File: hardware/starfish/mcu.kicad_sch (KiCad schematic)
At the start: 40 parts, among them SW301 RESET, SW302 BOOTSEL, U301 RP2040, U302 W25Q128JVS, Y301 12MHz

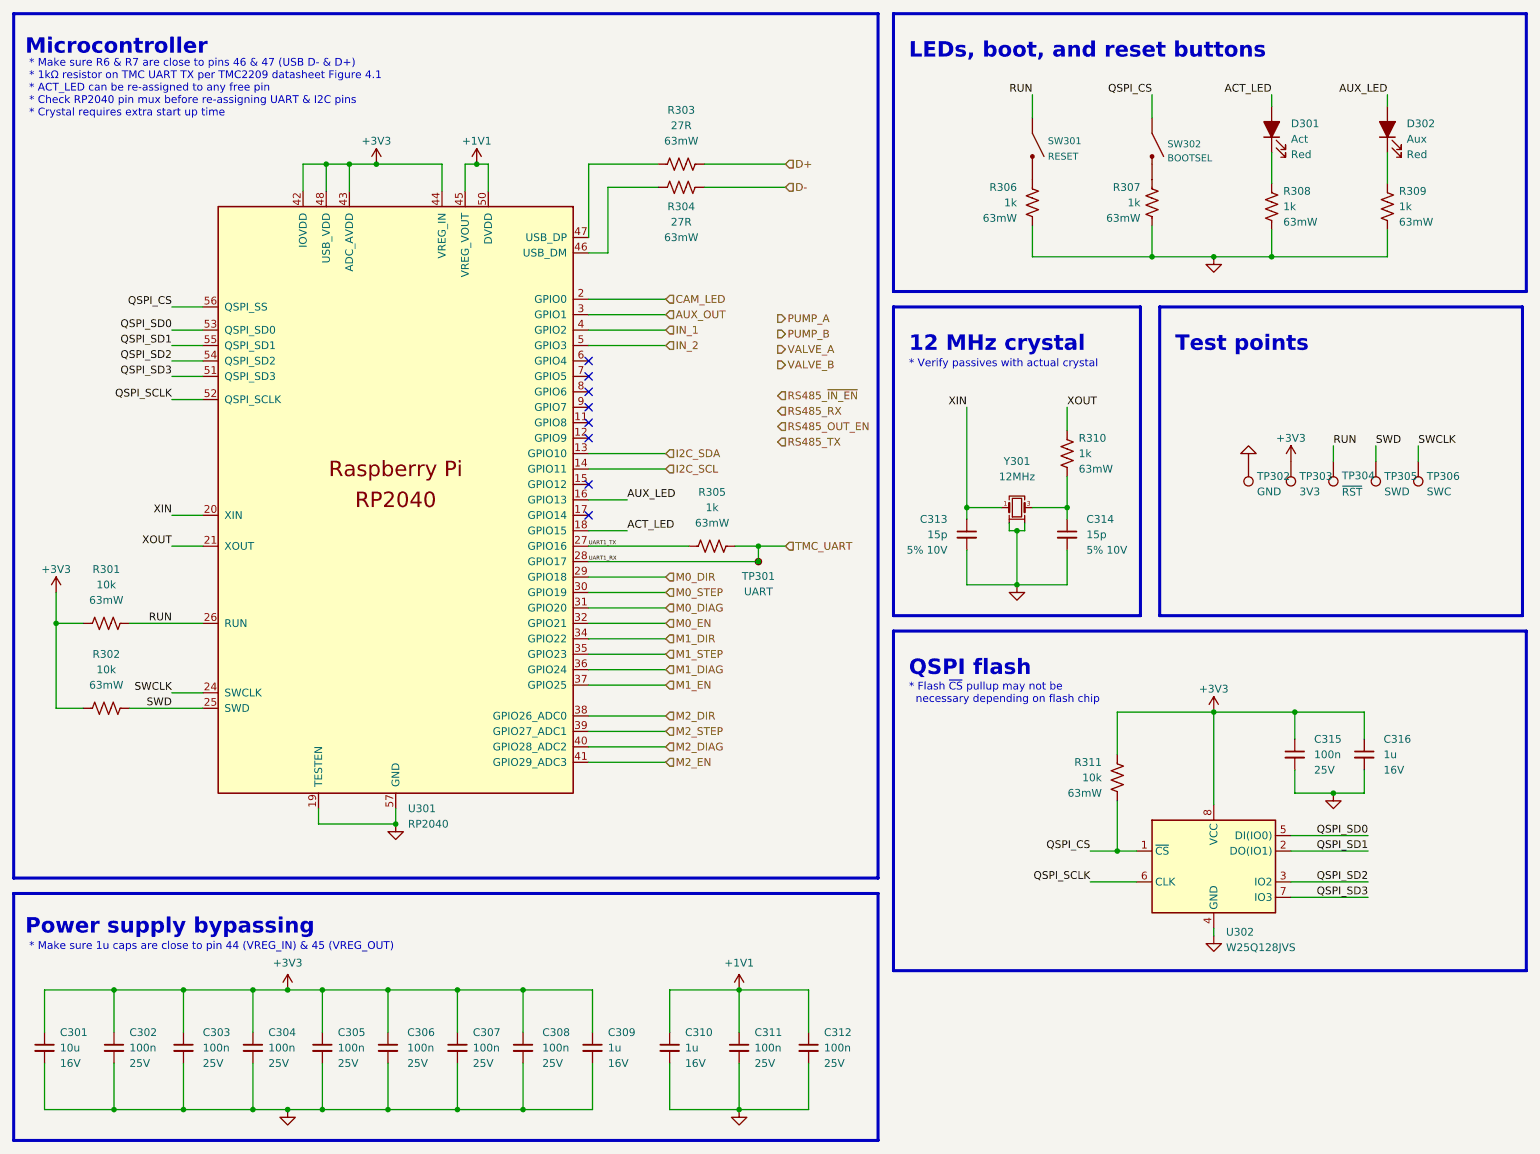
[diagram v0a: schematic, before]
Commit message: First pass at layout and routing
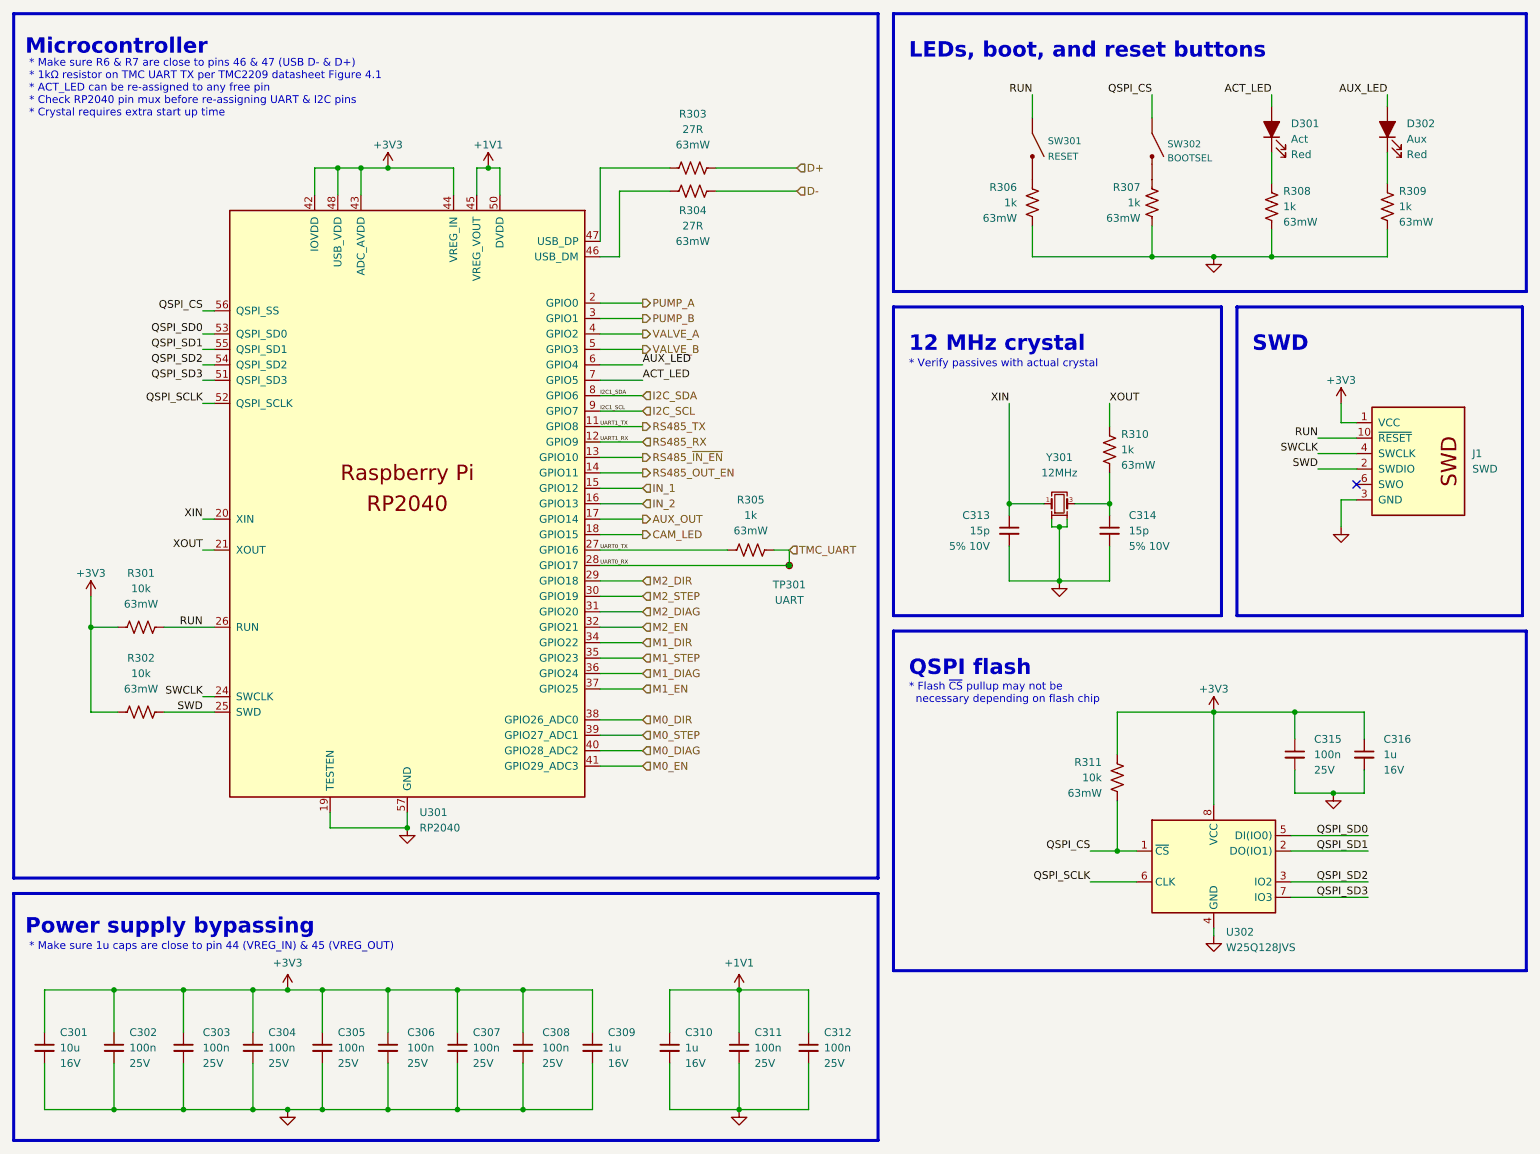
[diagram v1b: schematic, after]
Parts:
- removed TP302: GND, TestPoint:TestPoint_Pad_D1.0mm, symbol Connector:TestPoint
- removed TP303: 3V3, TestPoint:TestPoint_Pad_D1.0mm, symbol Connector:TestPoint
- removed TP304: ~{RST}, TestPoint:TestPoint_Pad_D1.0mm, symbol Connector:TestPoint
- removed TP305: SWD, TestPoint:TestPoint_Pad_D1.0mm, symbol Connector:TestPoint
- removed TP306: SWC, TestPoint:TestPoint_Pad_D1.0mm, symbol Connector:TestPoint
- added J1: SWD, winterbloom:Connector_Cortex_Debug_IDC_2x05_P1.27mm_Vertical_Shrouded_SMD, symbol winterbloom:Conn_SWD
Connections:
- net +3V3: now also J1.1 (VCC)
- net ACT_LED: now also U301.7 (GPIO5); no longer U301.18 (GPIO15)
- net AUX_LED: now also U301.6 (GPIO4); no longer U301.16 (GPIO13)
- net AUX_OUT: now also U301.17 (GPIO14); no longer U301.3 (GPIO1)
- net CAM_LED: now also U301.18 (GPIO15); no longer U301.2 (GPIO0)
- net GND: now also J1.3 (GND), J1.5 (GND), J1.9 (GNDDetect)
- net I2C_SCL: now also U301.9 (GPIO7); no longer U301.14 (GPIO11)
- net I2C_SDA: now also U301.8 (GPIO6); no longer U301.13 (GPIO10)
- net IN_1: now also U301.15 (GPIO12); no longer U301.4 (GPIO2)
- net IN_2: now also U301.16 (GPIO13); no longer U301.5 (GPIO3)
- net M0_DIAG: now also U301.40 (GPIO28_ADC2); no longer U301.31 (GPIO20)
- net M0_DIR: now also U301.38 (GPIO26_ADC0); no longer U301.29 (GPIO18)
- net M0_EN: now also U301.41 (GPIO29_ADC3); no longer U301.32 (GPIO21)
- net M0_STEP: now also U301.39 (GPIO27_ADC1); no longer U301.30 (GPIO19)
- net M2_DIAG: now also U301.31 (GPIO20); no longer U301.40 (GPIO28_ADC2)
- net M2_DIR: now also U301.29 (GPIO18); no longer U301.38 (GPIO26_ADC0)
- net M2_EN: now also U301.32 (GPIO21); no longer U301.41 (GPIO29_ADC3)
- net M2_STEP: now also U301.30 (GPIO19); no longer U301.39 (GPIO27_ADC1)
- net PUMP_A: now also U301.2 (GPIO0)
- net PUMP_B: now also U301.3 (GPIO1)
- net RS485_OUT_EN: now also U301.14 (GPIO11)
- net RS485_RX: now also U301.12 (GPIO9)
- net RS485_TX: now also U301.11 (GPIO8)
- net RS485_~{IN_EN}: now also U301.13 (GPIO10)
- net RUN: now also J1.10 (~{RESET})
- net SWCLK: now also J1.4 (SWCLK)
- net SWD: now also J1.2 (SWDIO)
- net TMC_UART: now also R305.1; no longer R305.2
- net VALVE_A: now also U301.4 (GPIO2)
- net VALVE_B: now also U301.5 (GPIO3)
- net UART1_TX renamed UART0_TX
- net UART0_TX: now also R305.2; no longer R305.1
- no-connect marks 8 -> 1
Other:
- note added: "SWD"
- note removed: "Test points"
- moved on the sheet: C313, C314, R301, R302, R303, R304, R305, R310, TP301, U301, Y301
